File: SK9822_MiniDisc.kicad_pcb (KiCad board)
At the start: 2 copper layers, 210 x 210 mm, 331 parts

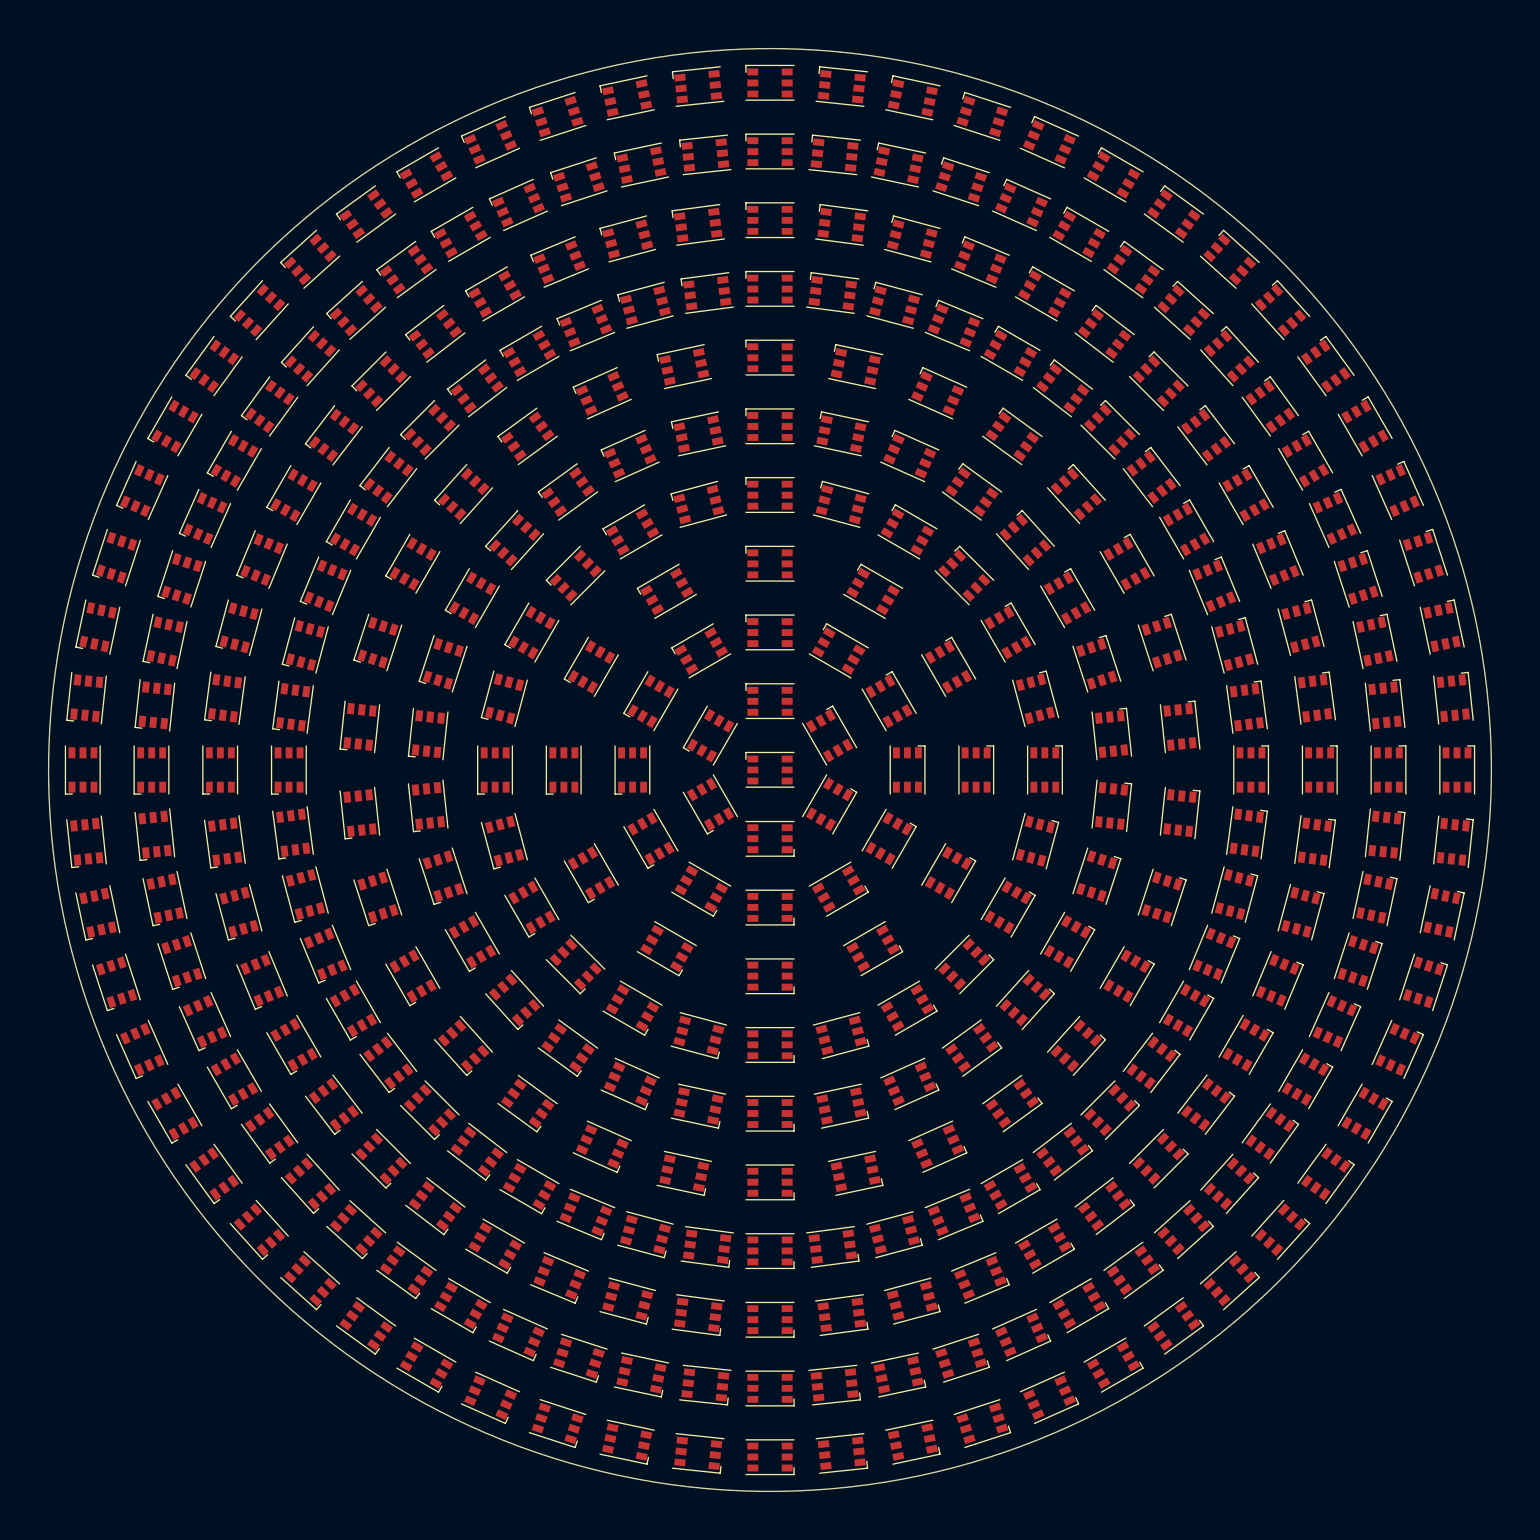
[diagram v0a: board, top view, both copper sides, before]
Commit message: Complete signal routing. Power needed
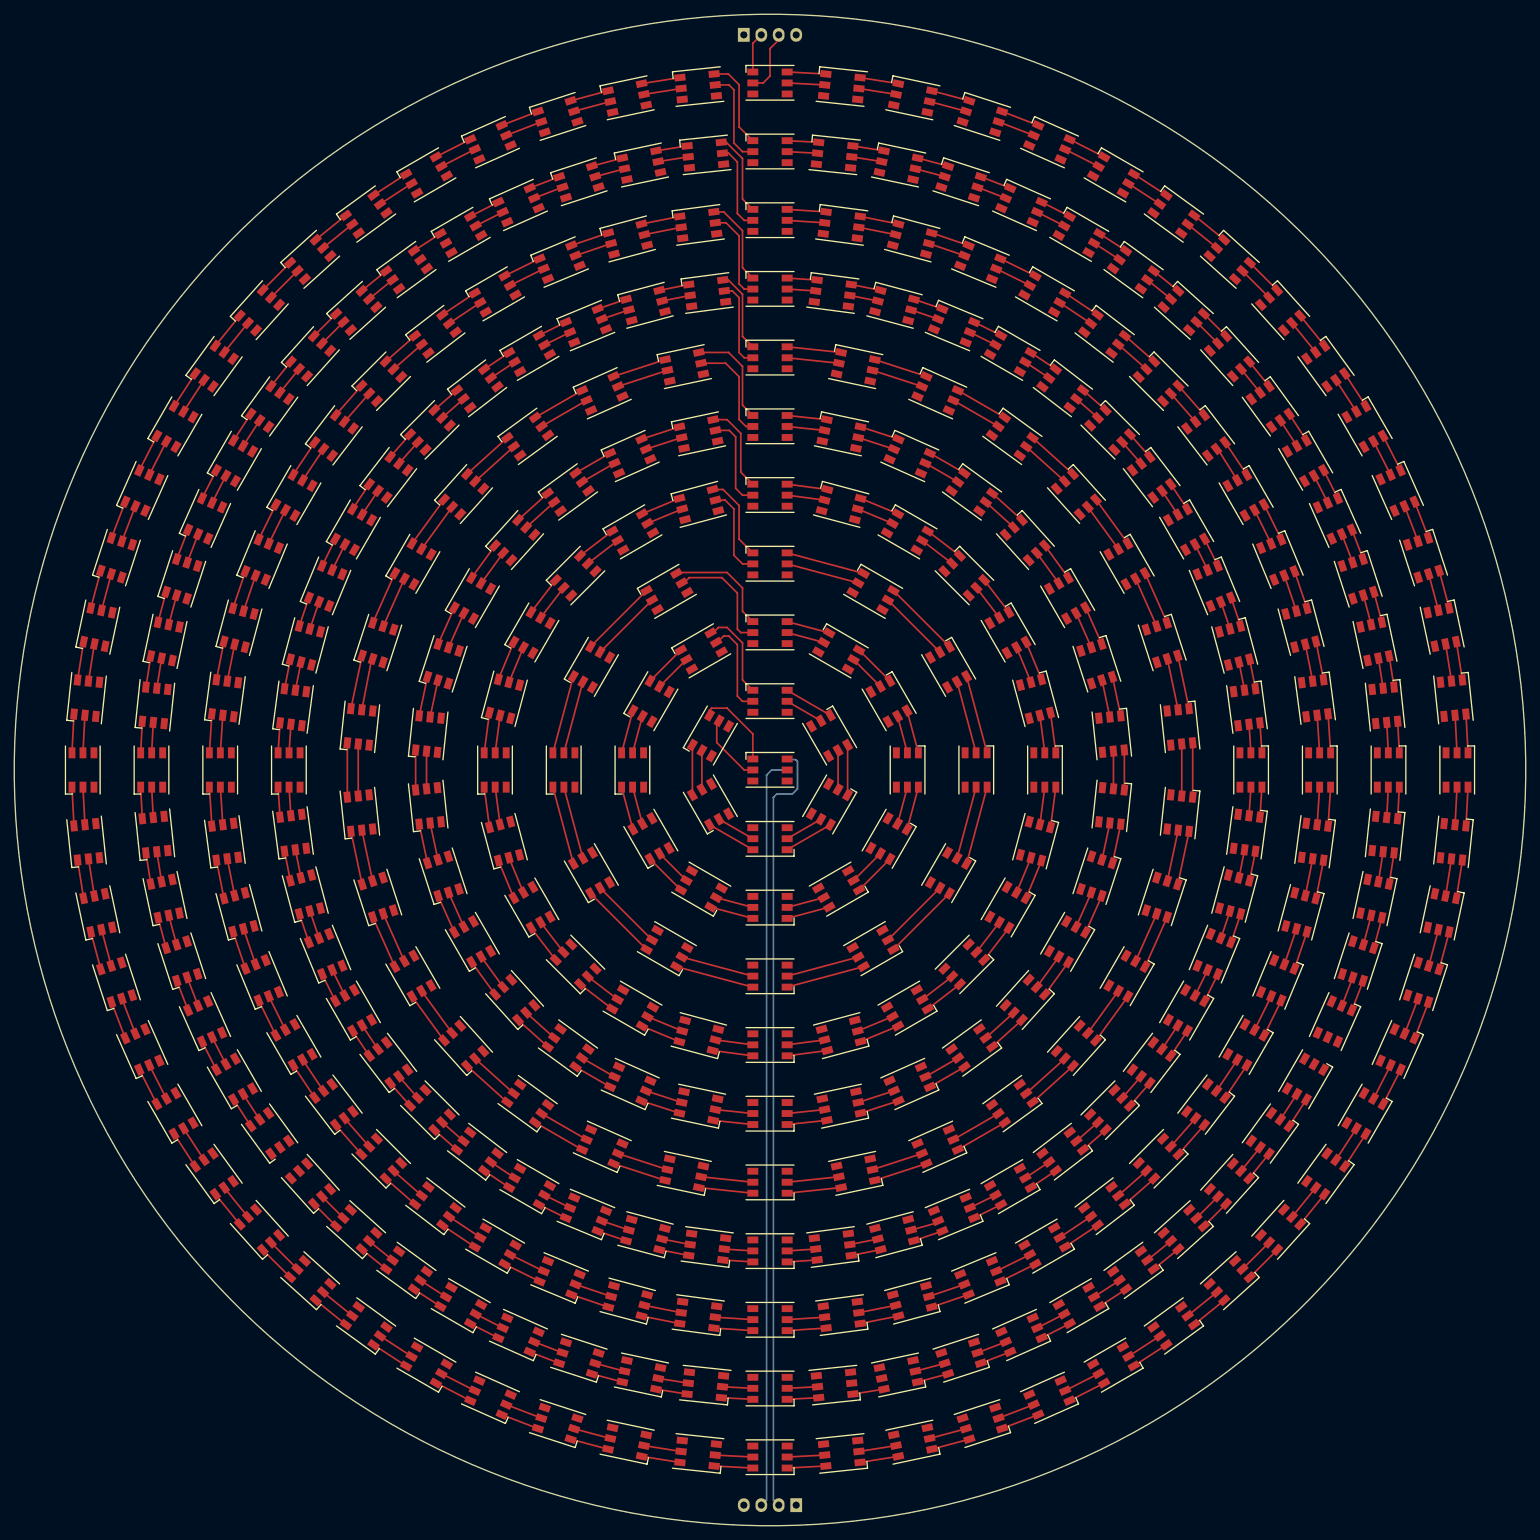
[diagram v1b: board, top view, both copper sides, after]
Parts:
- added P1: CONN_01X04, Conn:Angled_1x4, B.Cu at (300.0, 93.0)
- added P2: CONN_01X04, Conn:Angled_1x4, B.Cu at (300.0, 307.0)
- D1, D10, D100, D101, D102, D103, D104, D105, D106, D107, D108, D109, D11, D110, D111, D112, D113, D114, D115, D116, D117, D118, D119, D12, D120, D121, D122, D123, D124, D125, D126, D127, D128, D129, D13, D130, D131, D132, D133, D134, D135, D136, D137, D138, D139, D14, D140, D141, D142, D143, D144, D145, D146, D147, D148, D149, D15, D150, D151, D152, D153, D154, D155, D156, D157, D158, D159, D16, D160, D161, D162, D163, D164, D165, D166, D167, D168, D169, D17, D170, D171, D172, D173, D174, D175, D176, D177, D178, D179, D18, D180, D181, D182, D183, D184, D185, D186, D187, D188, D189, D19, D190, D191, D192, D193, D194, D195, D196, D197, D198, D199, D2, D20, D200, D201, D202, D203, D204, D205, D206, D207, D208, D209, D21, D210, D211, D212, D213, D214, D215, D216, D217, D218, D219, D22, D220, D221, D222, D223, D224, D225, D226, D227, D228, D229, D23, D230, D231, D232, D233, D234, D235, D236, D237, D238, D239, D24, D240, D241, D242, D243, D244, D245, D246, D247, D248, D249, D25, D250, D251, D252, D253, D254, D255, D256, D257, D258, D259, D26, D260, D261, D262, D263, D264, D265, D266, D267, D268, D269, D27, D270, D271, D272, D273, D274, D275, D276, D277, D278, D279, D28, D280, D281, D282, D283, D284, D285, D286, D287, D288, D289, D29, D290, D291, D292, D293, D294, D295, D296, D297, D298, D299, D3, D30, D300, D301, D302, D303, D304, D305, D306, D307, D308, D309, D31, D310, D311, D312, D313, D314, D315, D316, D317, D318, D319, D32, D320, D321, D322, D323, D324, D325, D326, D327, D328, D329, D33, D330, D331, D34, D35, D36, D37, D38, D39, D4, D40, D41, D42, D43, D44, D45, D46, D47, D48, D49, D5, D50, D51, D52, D53, D54, D55, D56, D57, D58, D59, D6, D60, D61, D62, D63, D64, D65, D66, D67, D68, D69, D7, D70, D71, D72, D73, D74, D75, D76, D77, D78, D79, D8, D80, D81, D82, D83, D84, D85, D86, D87, D88, D89, D9, D90, D91, D92, D93, D94, D95, D96, D97, D98, D99: value SK9822 -> APA102/SK9822
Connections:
- D1 pad 1: (no net) -> Net-(D1-Pad1)
- D1 pad 2: (no net) -> Net-(D1-Pad2)
- D1 pad 3: (no net) -> GND
- D1 pad 4: (no net) -> VCC
- D1 pad 5: (no net) -> Net-(D1-Pad5)
- D1 pad 6: (no net) -> Net-(D1-Pad6)
- D10 pad 1: (no net) -> Net-(D10-Pad1)
- D10 pad 2: (no net) -> Net-(D10-Pad2)
- D10 pad 3: (no net) -> GND
- D10 pad 4: (no net) -> VCC
- D10 pad 5: (no net) -> Net-(D10-Pad5)
- D10 pad 6: (no net) -> Net-(D10-Pad6)
- D100 pad 1: (no net) -> Net-(D100-Pad1)
- D100 pad 2: (no net) -> Net-(D100-Pad2)
- D100 pad 3: (no net) -> GND
- D100 pad 4: (no net) -> VCC
- D100 pad 5: (no net) -> Net-(D100-Pad5)
- D100 pad 6: (no net) -> Net-(D100-Pad6)
- D101 pad 1: (no net) -> Net-(D100-Pad6)
- D101 pad 2: (no net) -> Net-(D100-Pad5)
- D101 pad 3: (no net) -> GND
- D101 pad 4: (no net) -> VCC
- D101 pad 5: (no net) -> Net-(D101-Pad5)
- D101 pad 6: (no net) -> Net-(D101-Pad6)
- D102 pad 1: (no net) -> Net-(D101-Pad6)
- D102 pad 2: (no net) -> Net-(D101-Pad5)
- D102 pad 3: (no net) -> GND
- D102 pad 4: (no net) -> VCC
- D102 pad 5: (no net) -> Net-(D102-Pad5)
- D102 pad 6: (no net) -> Net-(D102-Pad6)
- D103 pad 1: (no net) -> Net-(D102-Pad6)
- D103 pad 2: (no net) -> Net-(D102-Pad5)
- D103 pad 3: (no net) -> GND
- D103 pad 4: (no net) -> VCC
- D103 pad 5: (no net) -> Net-(D103-Pad5)
- D103 pad 6: (no net) -> Net-(D103-Pad6)
- D104 pad 1: (no net) -> Net-(D103-Pad6)
- D104 pad 2: (no net) -> Net-(D103-Pad5)
- D104 pad 3: (no net) -> GND
- D104 pad 4: (no net) -> VCC
- D104 pad 5: (no net) -> Net-(D104-Pad5)
- D104 pad 6: (no net) -> Net-(D104-Pad6)
- D105 pad 1: (no net) -> Net-(D104-Pad6)
- D105 pad 2: (no net) -> Net-(D104-Pad5)
- D105 pad 3: (no net) -> GND
- D105 pad 4: (no net) -> VCC
- D105 pad 5: (no net) -> Net-(D105-Pad5)
- D105 pad 6: (no net) -> Net-(D105-Pad6)
- D106 pad 1: (no net) -> Net-(D105-Pad6)
- D106 pad 2: (no net) -> Net-(D105-Pad5)
- D106 pad 3: (no net) -> GND
- D106 pad 4: (no net) -> VCC
- D106 pad 5: (no net) -> Net-(D106-Pad5)
- D106 pad 6: (no net) -> Net-(D106-Pad6)
- D107 pad 1: (no net) -> Net-(D106-Pad6)
- D107 pad 2: (no net) -> Net-(D106-Pad5)
- D107 pad 3: (no net) -> GND
- D107 pad 4: (no net) -> VCC
- D107 pad 5: (no net) -> Net-(D107-Pad5)
- D107 pad 6: (no net) -> Net-(D107-Pad6)
- D108 pad 1: (no net) -> Net-(D107-Pad6)
- D108 pad 2: (no net) -> Net-(D107-Pad5)
- D108 pad 3: (no net) -> GND
- D108 pad 4: (no net) -> VCC
- D108 pad 5: (no net) -> Net-(D108-Pad5)
- D108 pad 6: (no net) -> Net-(D108-Pad6)
- D109 pad 1: (no net) -> Net-(D108-Pad6)
- D109 pad 2: (no net) -> Net-(D108-Pad5)
- D109 pad 3: (no net) -> GND
- D109 pad 4: (no net) -> VCC
- D109 pad 5: (no net) -> Net-(D109-Pad5)
- D109 pad 6: (no net) -> Net-(D109-Pad6)
- D11 pad 1: (no net) -> Net-(D10-Pad6)
- D11 pad 2: (no net) -> Net-(D10-Pad5)
- D11 pad 3: (no net) -> GND
- D11 pad 4: (no net) -> VCC
- D11 pad 5: (no net) -> Net-(D11-Pad5)
- D11 pad 6: (no net) -> Net-(D11-Pad6)
- D110 pad 1: (no net) -> Net-(D109-Pad6)
- D110 pad 2: (no net) -> Net-(D109-Pad5)
- D110 pad 3: (no net) -> GND
- D110 pad 4: (no net) -> VCC
- D110 pad 5: (no net) -> Net-(D110-Pad5)
- D110 pad 6: (no net) -> Net-(D110-Pad6)
- D111 pad 1: (no net) -> Net-(D110-Pad6)
- D111 pad 2: (no net) -> Net-(D110-Pad5)
- D111 pad 3: (no net) -> GND
- D111 pad 4: (no net) -> VCC
- D111 pad 5: (no net) -> Net-(D111-Pad5)
- D111 pad 6: (no net) -> Net-(D111-Pad6)
- D112 pad 1: (no net) -> Net-(D111-Pad6)
- D112 pad 2: (no net) -> Net-(D111-Pad5)
- D112 pad 3: (no net) -> GND
- D112 pad 4: (no net) -> VCC
- D112 pad 5: (no net) -> Net-(D112-Pad5)
- D112 pad 6: (no net) -> Net-(D112-Pad6)
- D113 pad 1: (no net) -> Net-(D112-Pad6)
- D113 pad 2: (no net) -> Net-(D112-Pad5)
- D113 pad 3: (no net) -> GND
- D113 pad 4: (no net) -> VCC
- D113 pad 5: (no net) -> Net-(D113-Pad5)
- D113 pad 6: (no net) -> Net-(D113-Pad6)
- D114 pad 1: (no net) -> Net-(D113-Pad6)
- D114 pad 2: (no net) -> Net-(D113-Pad5)
- D114 pad 3: (no net) -> GND
- D114 pad 4: (no net) -> VCC
- D114 pad 5: (no net) -> Net-(D114-Pad5)
- D114 pad 6: (no net) -> Net-(D114-Pad6)
- D115 pad 1: (no net) -> Net-(D114-Pad6)
- D115 pad 2: (no net) -> Net-(D114-Pad5)
- D115 pad 3: (no net) -> GND
- D115 pad 4: (no net) -> VCC
- D115 pad 5: (no net) -> Net-(D115-Pad5)
- D115 pad 6: (no net) -> Net-(D115-Pad6)
- D116 pad 1: (no net) -> Net-(D115-Pad6)
- D116 pad 2: (no net) -> Net-(D115-Pad5)
- D116 pad 3: (no net) -> GND
- D116 pad 4: (no net) -> VCC
- D116 pad 5: (no net) -> Net-(D116-Pad5)
- D116 pad 6: (no net) -> Net-(D116-Pad6)
- D117 pad 1: (no net) -> Net-(D116-Pad6)
- D117 pad 2: (no net) -> Net-(D116-Pad5)
- D117 pad 3: (no net) -> GND
- D117 pad 4: (no net) -> VCC
- D117 pad 5: (no net) -> Net-(D117-Pad5)
- D117 pad 6: (no net) -> Net-(D117-Pad6)
- D118 pad 1: (no net) -> Net-(D117-Pad6)
- D118 pad 2: (no net) -> Net-(D117-Pad5)
- D118 pad 3: (no net) -> GND
- D118 pad 4: (no net) -> VCC
- D118 pad 5: (no net) -> Net-(D118-Pad5)
- D118 pad 6: (no net) -> Net-(D118-Pad6)
- D119 pad 1: (no net) -> Net-(D118-Pad6)
- D119 pad 2: (no net) -> Net-(D118-Pad5)
- D119 pad 3: (no net) -> GND
- D119 pad 4: (no net) -> VCC
- D119 pad 5: (no net) -> Net-(D119-Pad5)
- D119 pad 6: (no net) -> Net-(D119-Pad6)
- D12 pad 1: (no net) -> Net-(D11-Pad6)
- D12 pad 2: (no net) -> Net-(D11-Pad5)
- D12 pad 3: (no net) -> GND
- D12 pad 4: (no net) -> VCC
- D12 pad 5: (no net) -> Net-(D12-Pad5)
- D12 pad 6: (no net) -> Net-(D12-Pad6)
- D120 pad 1: (no net) -> Net-(D119-Pad6)
- D120 pad 2: (no net) -> Net-(D119-Pad5)
- D120 pad 3: (no net) -> GND
- D120 pad 4: (no net) -> VCC
- D120 pad 5: (no net) -> Net-(D120-Pad5)
- D120 pad 6: (no net) -> Net-(D120-Pad6)
- D121 pad 1: (no net) -> Net-(D120-Pad6)
- D121 pad 2: (no net) -> Net-(D120-Pad5)
- D121 pad 3: (no net) -> GND
- D121 pad 4: (no net) -> VCC
- D121 pad 5: (no net) -> Net-(D121-Pad5)
- D121 pad 6: (no net) -> Net-(D121-Pad6)
- D122 pad 1: (no net) -> Net-(D121-Pad6)
- D122 pad 2: (no net) -> Net-(D121-Pad5)
- D122 pad 3: (no net) -> GND
- D122 pad 4: (no net) -> VCC
- D122 pad 5: (no net) -> Net-(D122-Pad5)
- D122 pad 6: (no net) -> Net-(D122-Pad6)
- D123 pad 1: (no net) -> Net-(D122-Pad6)
- D123 pad 2: (no net) -> Net-(D122-Pad5)
- D123 pad 3: (no net) -> GND
- D123 pad 4: (no net) -> VCC
- D123 pad 5: (no net) -> Net-(D123-Pad5)
- D123 pad 6: (no net) -> Net-(D123-Pad6)
- D124 pad 1: (no net) -> Net-(D123-Pad6)
- D124 pad 2: (no net) -> Net-(D123-Pad5)
- D124 pad 3: (no net) -> GND
- D124 pad 4: (no net) -> VCC
- D124 pad 5: (no net) -> Net-(D124-Pad5)
- D124 pad 6: (no net) -> Net-(D124-Pad6)
- D125 pad 1: (no net) -> Net-(D124-Pad6)
- D125 pad 2: (no net) -> Net-(D124-Pad5)
- D125 pad 3: (no net) -> GND
- D125 pad 4: (no net) -> VCC
- D125 pad 5: (no net) -> Net-(D125-Pad5)
- D125 pad 6: (no net) -> Net-(D125-Pad6)
- D126 pad 1: (no net) -> Net-(D125-Pad6)
- D126 pad 2: (no net) -> Net-(D125-Pad5)
- D126 pad 3: (no net) -> GND
- D126 pad 4: (no net) -> VCC
- D126 pad 5: (no net) -> Net-(D126-Pad5)
- D126 pad 6: (no net) -> Net-(D126-Pad6)
- D127 pad 1: (no net) -> Net-(D126-Pad6)
- D127 pad 2: (no net) -> Net-(D126-Pad5)
- D127 pad 3: (no net) -> GND
- D127 pad 4: (no net) -> VCC
- D127 pad 5: (no net) -> Net-(D127-Pad5)
- D127 pad 6: (no net) -> Net-(D127-Pad6)
- D128 pad 1: (no net) -> Net-(D127-Pad6)
- D128 pad 2: (no net) -> Net-(D127-Pad5)
- D128 pad 3: (no net) -> GND
- D128 pad 4: (no net) -> VCC
- D128 pad 5: (no net) -> Net-(D128-Pad5)
- D128 pad 6: (no net) -> Net-(D128-Pad6)
- D129 pad 1: (no net) -> Net-(D128-Pad6)
- D129 pad 2: (no net) -> Net-(D128-Pad5)
- D129 pad 3: (no net) -> GND
- D129 pad 4: (no net) -> VCC
- D129 pad 5: (no net) -> Net-(D129-Pad5)
- D129 pad 6: (no net) -> Net-(D129-Pad6)
- D13 pad 1: (no net) -> Net-(D12-Pad6)
- D13 pad 2: (no net) -> Net-(D12-Pad5)
- D13 pad 3: (no net) -> GND
- D13 pad 4: (no net) -> VCC
- D13 pad 5: (no net) -> Net-(D13-Pad5)
- D13 pad 6: (no net) -> Net-(D13-Pad6)
- D130 pad 1: (no net) -> Net-(D129-Pad6)
- D130 pad 2: (no net) -> Net-(D129-Pad5)
- D130 pad 3: (no net) -> GND
- D130 pad 4: (no net) -> VCC
- D130 pad 5: (no net) -> Net-(D130-Pad5)
- D130 pad 6: (no net) -> Net-(D130-Pad6)
- D131 pad 1: (no net) -> Net-(D130-Pad6)
- D131 pad 2: (no net) -> Net-(D130-Pad5)
- D131 pad 3: (no net) -> GND
- D131 pad 4: (no net) -> VCC
- D131 pad 5: (no net) -> Net-(D131-Pad5)
- D131 pad 6: (no net) -> Net-(D131-Pad6)
- D132 pad 1: (no net) -> Net-(D131-Pad6)
- D132 pad 2: (no net) -> Net-(D131-Pad5)
- D132 pad 3: (no net) -> GND
- D132 pad 4: (no net) -> VCC
- D132 pad 5: (no net) -> Net-(D132-Pad5)
- D132 pad 6: (no net) -> Net-(D132-Pad6)
- D133 pad 1: (no net) -> Net-(D132-Pad6)
- D133 pad 2: (no net) -> Net-(D132-Pad5)
- D133 pad 3: (no net) -> GND
- D133 pad 4: (no net) -> VCC
- D133 pad 5: (no net) -> Net-(D133-Pad5)
- D133 pad 6: (no net) -> Net-(D133-Pad6)
- D134 pad 1: (no net) -> Net-(D133-Pad6)
- D134 pad 2: (no net) -> Net-(D133-Pad5)
- D134 pad 3: (no net) -> GND
- D134 pad 4: (no net) -> VCC
- D134 pad 5: (no net) -> Net-(D134-Pad5)
- D134 pad 6: (no net) -> Net-(D134-Pad6)
- D135 pad 1: (no net) -> Net-(D134-Pad6)
- D135 pad 2: (no net) -> Net-(D134-Pad5)
- D135 pad 3: (no net) -> GND
- D135 pad 4: (no net) -> VCC
- D135 pad 5: (no net) -> Net-(D135-Pad5)
- D135 pad 6: (no net) -> Net-(D135-Pad6)
- D136 pad 1: (no net) -> Net-(D135-Pad6)
- D136 pad 2: (no net) -> Net-(D135-Pad5)
- D136 pad 3: (no net) -> GND
- D136 pad 4: (no net) -> VCC
- D136 pad 5: (no net) -> Net-(D136-Pad5)
- D136 pad 6: (no net) -> Net-(D136-Pad6)
- D137 pad 1: (no net) -> Net-(D136-Pad6)
- D137 pad 2: (no net) -> Net-(D136-Pad5)
- D137 pad 3: (no net) -> GND
- D137 pad 4: (no net) -> VCC
- D137 pad 5: (no net) -> Net-(D137-Pad5)
- D137 pad 6: (no net) -> Net-(D137-Pad6)
- D138 pad 1: (no net) -> Net-(D137-Pad6)
- D138 pad 2: (no net) -> Net-(D137-Pad5)
- D138 pad 3: (no net) -> GND
- D138 pad 4: (no net) -> VCC
- D138 pad 5: (no net) -> Net-(D138-Pad5)
- D138 pad 6: (no net) -> Net-(D138-Pad6)
- D139 pad 1: (no net) -> Net-(D138-Pad6)
- D139 pad 2: (no net) -> Net-(D138-Pad5)
- D139 pad 3: (no net) -> GND
- D139 pad 4: (no net) -> VCC
- D139 pad 5: (no net) -> Net-(D139-Pad5)
- D139 pad 6: (no net) -> Net-(D139-Pad6)
- D14 pad 1: (no net) -> Net-(D13-Pad6)
- D14 pad 2: (no net) -> Net-(D13-Pad5)
- D14 pad 3: (no net) -> GND
- D14 pad 4: (no net) -> VCC
- D14 pad 5: (no net) -> Net-(D14-Pad5)
- D14 pad 6: (no net) -> Net-(D14-Pad6)
- D140 pad 1: (no net) -> Net-(D139-Pad6)
- D140 pad 2: (no net) -> Net-(D139-Pad5)
- D140 pad 3: (no net) -> GND
- D140 pad 4: (no net) -> VCC
- D140 pad 5: (no net) -> Net-(D140-Pad5)
- D140 pad 6: (no net) -> Net-(D140-Pad6)
- D141 pad 1: (no net) -> Net-(D140-Pad6)
- D141 pad 2: (no net) -> Net-(D140-Pad5)
- D141 pad 3: (no net) -> GND
- D141 pad 4: (no net) -> VCC
- D141 pad 5: (no net) -> Net-(D141-Pad5)
- D141 pad 6: (no net) -> Net-(D141-Pad6)
- D142 pad 1: (no net) -> Net-(D141-Pad6)
- D142 pad 2: (no net) -> Net-(D141-Pad5)
- D142 pad 3: (no net) -> GND
- D142 pad 4: (no net) -> VCC
- D142 pad 5: (no net) -> Net-(D142-Pad5)
- D142 pad 6: (no net) -> Net-(D142-Pad6)
- D143 pad 1: (no net) -> Net-(D142-Pad6)
- D143 pad 2: (no net) -> Net-(D142-Pad5)
- D143 pad 3: (no net) -> GND
- D143 pad 4: (no net) -> VCC
- D143 pad 5: (no net) -> Net-(D143-Pad5)
- D143 pad 6: (no net) -> Net-(D143-Pad6)
- D144 pad 1: (no net) -> Net-(D143-Pad6)
- D144 pad 2: (no net) -> Net-(D143-Pad5)
- D144 pad 3: (no net) -> GND
- D144 pad 4: (no net) -> VCC
- D144 pad 5: (no net) -> Net-(D144-Pad5)
- D144 pad 6: (no net) -> Net-(D144-Pad6)
- D145 pad 1: (no net) -> Net-(D144-Pad6)
- D145 pad 2: (no net) -> Net-(D144-Pad5)
- D145 pad 3: (no net) -> GND
- D145 pad 4: (no net) -> VCC
- D145 pad 5: (no net) -> Net-(D145-Pad5)
- D145 pad 6: (no net) -> Net-(D145-Pad6)
- D146 pad 1: (no net) -> Net-(D145-Pad6)
- D146 pad 2: (no net) -> Net-(D145-Pad5)
- D146 pad 3: (no net) -> GND
- D146 pad 4: (no net) -> VCC
- D146 pad 5: (no net) -> Net-(D146-Pad5)
- D146 pad 6: (no net) -> Net-(D146-Pad6)
- D147 pad 1: (no net) -> Net-(D146-Pad6)
- D147 pad 2: (no net) -> Net-(D146-Pad5)
- D147 pad 3: (no net) -> GND
- D147 pad 4: (no net) -> VCC
- D147 pad 5: (no net) -> Net-(D147-Pad5)
- D147 pad 6: (no net) -> Net-(D147-Pad6)
- D148 pad 1: (no net) -> Net-(D147-Pad6)
- D148 pad 2: (no net) -> Net-(D147-Pad5)
- D148 pad 3: (no net) -> GND
- D148 pad 4: (no net) -> VCC
- D148 pad 5: (no net) -> Net-(D148-Pad5)
- D148 pad 6: (no net) -> Net-(D148-Pad6)
- D149 pad 1: (no net) -> Net-(D148-Pad6)
- D149 pad 2: (no net) -> Net-(D148-Pad5)
- D149 pad 3: (no net) -> GND
- D149 pad 4: (no net) -> VCC
- D149 pad 5: (no net) -> Net-(D149-Pad5)
- D149 pad 6: (no net) -> Net-(D149-Pad6)
- D15 pad 1: (no net) -> Net-(D14-Pad6)
- D15 pad 2: (no net) -> Net-(D14-Pad5)
- D15 pad 3: (no net) -> GND
- D15 pad 4: (no net) -> VCC
- D15 pad 5: (no net) -> Net-(D15-Pad5)
- D15 pad 6: (no net) -> Net-(D15-Pad6)
- D150 pad 1: (no net) -> Net-(D149-Pad6)
- D150 pad 2: (no net) -> Net-(D149-Pad5)
- D150 pad 3: (no net) -> GND
- D150 pad 4: (no net) -> VCC
- D150 pad 5: (no net) -> Net-(D150-Pad5)
- D150 pad 6: (no net) -> Net-(D150-Pad6)
- D151 pad 1: (no net) -> Net-(D150-Pad6)
- D151 pad 2: (no net) -> Net-(D150-Pad5)
- D151 pad 3: (no net) -> GND
- D151 pad 4: (no net) -> VCC
- D151 pad 5: (no net) -> Net-(D151-Pad5)
- D151 pad 6: (no net) -> Net-(D151-Pad6)
- D152 pad 1: (no net) -> Net-(D151-Pad6)
- D152 pad 2: (no net) -> Net-(D151-Pad5)
- D152 pad 3: (no net) -> GND
- D152 pad 4: (no net) -> VCC
- D152 pad 5: (no net) -> Net-(D152-Pad5)
- D152 pad 6: (no net) -> Net-(D152-Pad6)
- D153 pad 1: (no net) -> Net-(D152-Pad6)
- D153 pad 2: (no net) -> Net-(D152-Pad5)
- D153 pad 3: (no net) -> GND
- D153 pad 4: (no net) -> VCC
- D153 pad 5: (no net) -> Net-(D153-Pad5)
- D153 pad 6: (no net) -> Net-(D153-Pad6)
- D154 pad 1: (no net) -> Net-(D153-Pad6)
- D154 pad 2: (no net) -> Net-(D153-Pad5)
- D154 pad 3: (no net) -> GND
- D154 pad 4: (no net) -> VCC
- D154 pad 5: (no net) -> Net-(D154-Pad5)
- D154 pad 6: (no net) -> Net-(D154-Pad6)
- D155 pad 1: (no net) -> Net-(D154-Pad6)
- D155 pad 2: (no net) -> Net-(D154-Pad5)
- D155 pad 3: (no net) -> GND
- D155 pad 4: (no net) -> VCC
- D155 pad 5: (no net) -> Net-(D155-Pad5)
- D155 pad 6: (no net) -> Net-(D155-Pad6)
- D156 pad 1: (no net) -> Net-(D155-Pad6)
- D156 pad 2: (no net) -> Net-(D155-Pad5)
- D156 pad 3: (no net) -> GND
- D156 pad 4: (no net) -> VCC
- D156 pad 5: (no net) -> Net-(D156-Pad5)
- D156 pad 6: (no net) -> Net-(D156-Pad6)
- D157 pad 1: (no net) -> Net-(D156-Pad6)
- D157 pad 2: (no net) -> Net-(D156-Pad5)
- D157 pad 3: (no net) -> GND
- D157 pad 4: (no net) -> VCC
- D157 pad 5: (no net) -> Net-(D157-Pad5)
- D157 pad 6: (no net) -> Net-(D157-Pad6)
- D158 pad 1: (no net) -> Net-(D157-Pad6)
- D158 pad 2: (no net) -> Net-(D157-Pad5)
- D158 pad 3: (no net) -> GND
- D158 pad 4: (no net) -> VCC
- D158 pad 5: (no net) -> Net-(D158-Pad5)
- D158 pad 6: (no net) -> Net-(D158-Pad6)
- D159 pad 1: (no net) -> Net-(D158-Pad6)
- D159 pad 2: (no net) -> Net-(D158-Pad5)
- D159 pad 3: (no net) -> GND
- D159 pad 4: (no net) -> VCC
- D159 pad 5: (no net) -> Net-(D159-Pad5)
- D159 pad 6: (no net) -> Net-(D159-Pad6)
- D16 pad 1: (no net) -> Net-(D15-Pad6)
- D16 pad 2: (no net) -> Net-(D15-Pad5)
- D16 pad 3: (no net) -> GND
- D16 pad 4: (no net) -> VCC
- D16 pad 5: (no net) -> Net-(D16-Pad5)
- D16 pad 6: (no net) -> Net-(D16-Pad6)
- D160 pad 1: (no net) -> Net-(D159-Pad6)
- D160 pad 2: (no net) -> Net-(D159-Pad5)
- D160 pad 3: (no net) -> GND
- D160 pad 4: (no net) -> VCC
- D160 pad 5: (no net) -> Net-(D160-Pad5)
- D160 pad 6: (no net) -> Net-(D160-Pad6)
- D161 pad 1: (no net) -> Net-(D160-Pad6)
- D161 pad 2: (no net) -> Net-(D160-Pad5)
- D161 pad 3: (no net) -> GND
- D161 pad 4: (no net) -> VCC
- D161 pad 5: (no net) -> Net-(D161-Pad5)
- D161 pad 6: (no net) -> Net-(D161-Pad6)
- D162 pad 1: (no net) -> Net-(D161-Pad6)
- D162 pad 2: (no net) -> Net-(D161-Pad5)
- D162 pad 3: (no net) -> GND
- D162 pad 4: (no net) -> VCC
- D162 pad 5: (no net) -> Net-(D162-Pad5)
- D162 pad 6: (no net) -> Net-(D162-Pad6)
- D163 pad 1: (no net) -> Net-(D162-Pad6)
- D163 pad 2: (no net) -> Net-(D162-Pad5)
- D163 pad 3: (no net) -> GND
- D163 pad 4: (no net) -> VCC
- D163 pad 5: (no net) -> Net-(D163-Pad5)
- D163 pad 6: (no net) -> Net-(D163-Pad6)
- D164 pad 1: (no net) -> Net-(D163-Pad6)
- D164 pad 2: (no net) -> Net-(D163-Pad5)
- D164 pad 3: (no net) -> GND
- D164 pad 4: (no net) -> VCC
- D164 pad 5: (no net) -> Net-(D164-Pad5)
- D164 pad 6: (no net) -> Net-(D164-Pad6)
- D165 pad 1: (no net) -> Net-(D164-Pad6)
- D165 pad 2: (no net) -> Net-(D164-Pad5)
- D165 pad 3: (no net) -> GND
- D165 pad 4: (no net) -> VCC
- D165 pad 5: (no net) -> Net-(D165-Pad5)
- D165 pad 6: (no net) -> Net-(D165-Pad6)
- D166 pad 1: (no net) -> Net-(D165-Pad6)
- D166 pad 2: (no net) -> Net-(D165-Pad5)
- D166 pad 3: (no net) -> GND
- D166 pad 4: (no net) -> VCC
- D166 pad 5: (no net) -> Net-(D166-Pad5)
- D166 pad 6: (no net) -> Net-(D166-Pad6)
- D167 pad 1: (no net) -> Net-(D166-Pad6)
- D167 pad 2: (no net) -> Net-(D166-Pad5)
- D167 pad 3: (no net) -> GND
- D167 pad 4: (no net) -> VCC
- D167 pad 5: (no net) -> Net-(D167-Pad5)
- D167 pad 6: (no net) -> Net-(D167-Pad6)
- D168 pad 1: (no net) -> Net-(D167-Pad6)
- D168 pad 2: (no net) -> Net-(D167-Pad5)
- D168 pad 3: (no net) -> GND
- D168 pad 4: (no net) -> VCC
- D168 pad 5: (no net) -> Net-(D168-Pad5)
- D168 pad 6: (no net) -> Net-(D168-Pad6)
- D169 pad 1: (no net) -> Net-(D168-Pad6)
- D169 pad 2: (no net) -> Net-(D168-Pad5)
- D169 pad 3: (no net) -> GND
- D169 pad 4: (no net) -> VCC
- D169 pad 5: (no net) -> Net-(D169-Pad5)
- D169 pad 6: (no net) -> Net-(D169-Pad6)
- D17 pad 1: (no net) -> Net-(D16-Pad6)
- D17 pad 2: (no net) -> Net-(D16-Pad5)
- D17 pad 3: (no net) -> GND
- D17 pad 4: (no net) -> VCC
- D17 pad 5: (no net) -> Net-(D17-Pad5)
- D17 pad 6: (no net) -> Net-(D17-Pad6)
- D170 pad 1: (no net) -> Net-(D169-Pad6)
- D170 pad 2: (no net) -> Net-(D169-Pad5)
- D170 pad 3: (no net) -> GND
- D170 pad 4: (no net) -> VCC
- D170 pad 5: (no net) -> Net-(D170-Pad5)
- D170 pad 6: (no net) -> Net-(D170-Pad6)
- D171 pad 1: (no net) -> Net-(D170-Pad6)
- D171 pad 2: (no net) -> Net-(D170-Pad5)
- D171 pad 3: (no net) -> GND
- D171 pad 4: (no net) -> VCC
- D171 pad 5: (no net) -> Net-(D171-Pad5)
- D171 pad 6: (no net) -> Net-(D171-Pad6)
- D172 pad 1: (no net) -> Net-(D171-Pad6)
- D172 pad 2: (no net) -> Net-(D171-Pad5)
- D172 pad 3: (no net) -> GND
- D172 pad 4: (no net) -> VCC
- D172 pad 5: (no net) -> Net-(D172-Pad5)
- D172 pad 6: (no net) -> Net-(D172-Pad6)
- D173 pad 1: (no net) -> Net-(D172-Pad6)
- D173 pad 2: (no net) -> Net-(D172-Pad5)
- D173 pad 3: (no net) -> GND
- D173 pad 4: (no net) -> VCC
- D173 pad 5: (no net) -> Net-(D173-Pad5)
- D173 pad 6: (no net) -> Net-(D173-Pad6)
- D174 pad 1: (no net) -> Net-(D173-Pad6)
- D174 pad 2: (no net) -> Net-(D173-Pad5)
- D174 pad 3: (no net) -> GND
- D174 pad 4: (no net) -> VCC
- D174 pad 5: (no net) -> Net-(D174-Pad5)
- D174 pad 6: (no net) -> Net-(D174-Pad6)
- D175 pad 1: (no net) -> Net-(D174-Pad6)
- D175 pad 2: (no net) -> Net-(D174-Pad5)
- D175 pad 3: (no net) -> GND
- D175 pad 4: (no net) -> VCC
- D175 pad 5: (no net) -> Net-(D175-Pad5)
- D175 pad 6: (no net) -> Net-(D175-Pad6)
- D176 pad 1: (no net) -> Net-(D175-Pad6)
- D176 pad 2: (no net) -> Net-(D175-Pad5)
- D176 pad 3: (no net) -> GND
- D176 pad 4: (no net) -> VCC
- D176 pad 5: (no net) -> Net-(D176-Pad5)
- D176 pad 6: (no net) -> Net-(D176-Pad6)
- D177 pad 1: (no net) -> Net-(D176-Pad6)
- D177 pad 2: (no net) -> Net-(D176-Pad5)
- D177 pad 3: (no net) -> GND
- D177 pad 4: (no net) -> VCC
- D177 pad 5: (no net) -> Net-(D177-Pad5)
- D177 pad 6: (no net) -> Net-(D177-Pad6)
- D178 pad 1: (no net) -> Net-(D177-Pad6)
- D178 pad 2: (no net) -> Net-(D177-Pad5)
- D178 pad 3: (no net) -> GND
- D178 pad 4: (no net) -> VCC
- D178 pad 5: (no net) -> Net-(D178-Pad5)
- D178 pad 6: (no net) -> Net-(D178-Pad6)
- D179 pad 1: (no net) -> Net-(D178-Pad6)
- D179 pad 2: (no net) -> Net-(D178-Pad5)
- D179 pad 3: (no net) -> GND
- D179 pad 4: (no net) -> VCC
- D179 pad 5: (no net) -> Net-(D179-Pad5)
- D179 pad 6: (no net) -> Net-(D179-Pad6)
- D18 pad 1: (no net) -> Net-(D17-Pad6)
- D18 pad 2: (no net) -> Net-(D17-Pad5)
- D18 pad 3: (no net) -> GND
- D18 pad 4: (no net) -> VCC
- D18 pad 5: (no net) -> Net-(D18-Pad5)
- D18 pad 6: (no net) -> Net-(D18-Pad6)
- D180 pad 1: (no net) -> Net-(D179-Pad6)
- D180 pad 2: (no net) -> Net-(D179-Pad5)
- D180 pad 3: (no net) -> GND
- D180 pad 4: (no net) -> VCC
- D180 pad 5: (no net) -> Net-(D180-Pad5)
- D180 pad 6: (no net) -> Net-(D180-Pad6)
- D181 pad 1: (no net) -> Net-(D180-Pad6)
- D181 pad 2: (no net) -> Net-(D180-Pad5)
- D181 pad 3: (no net) -> GND
- D181 pad 4: (no net) -> VCC
- D181 pad 5: (no net) -> Net-(D181-Pad5)
- D181 pad 6: (no net) -> Net-(D181-Pad6)
- D182 pad 1: (no net) -> Net-(D181-Pad6)
- D182 pad 2: (no net) -> Net-(D181-Pad5)
- D182 pad 3: (no net) -> GND
- D182 pad 4: (no net) -> VCC
- D182 pad 5: (no net) -> Net-(D182-Pad5)
- D182 pad 6: (no net) -> Net-(D182-Pad6)
- D183 pad 1: (no net) -> Net-(D182-Pad6)
- D183 pad 2: (no net) -> Net-(D182-Pad5)
- D183 pad 3: (no net) -> GND
- D183 pad 4: (no net) -> VCC
- D183 pad 5: (no net) -> Net-(D183-Pad5)
- D183 pad 6: (no net) -> Net-(D183-Pad6)
- D184 pad 1: (no net) -> Net-(D183-Pad6)
- D184 pad 2: (no net) -> Net-(D183-Pad5)
- D184 pad 3: (no net) -> GND
- D184 pad 4: (no net) -> VCC
- D184 pad 5: (no net) -> Net-(D184-Pad5)
- D184 pad 6: (no net) -> Net-(D184-Pad6)
- D185 pad 1: (no net) -> Net-(D184-Pad6)
- D185 pad 2: (no net) -> Net-(D184-Pad5)
- D185 pad 3: (no net) -> GND
- D185 pad 4: (no net) -> VCC
- D185 pad 5: (no net) -> Net-(D185-Pad5)
- D185 pad 6: (no net) -> Net-(D185-Pad6)
- D186 pad 1: (no net) -> Net-(D185-Pad6)
- D186 pad 2: (no net) -> Net-(D185-Pad5)
- D186 pad 3: (no net) -> GND
- D186 pad 4: (no net) -> VCC
- D186 pad 5: (no net) -> Net-(D186-Pad5)
- D186 pad 6: (no net) -> Net-(D186-Pad6)
- D187 pad 1: (no net) -> Net-(D186-Pad6)
- D187 pad 2: (no net) -> Net-(D186-Pad5)
- D187 pad 3: (no net) -> GND
- D187 pad 4: (no net) -> VCC
- D187 pad 5: (no net) -> Net-(D187-Pad5)
- D187 pad 6: (no net) -> Net-(D187-Pad6)
- D188 pad 1: (no net) -> Net-(D187-Pad6)
- D188 pad 2: (no net) -> Net-(D187-Pad5)
- D188 pad 3: (no net) -> GND
- D188 pad 4: (no net) -> VCC
- D188 pad 5: (no net) -> Net-(D188-Pad5)
- D188 pad 6: (no net) -> Net-(D188-Pad6)
- D189 pad 1: (no net) -> Net-(D188-Pad6)
- D189 pad 2: (no net) -> Net-(D188-Pad5)
- D189 pad 3: (no net) -> GND
- D189 pad 4: (no net) -> VCC
- D189 pad 5: (no net) -> Net-(D189-Pad5)
- D189 pad 6: (no net) -> Net-(D189-Pad6)
- D19 pad 1: (no net) -> Net-(D18-Pad6)
- D19 pad 2: (no net) -> Net-(D18-Pad5)
- D19 pad 3: (no net) -> GND
- D19 pad 4: (no net) -> VCC
- D19 pad 5: (no net) -> Net-(D19-Pad5)
- D19 pad 6: (no net) -> Net-(D19-Pad6)
- D190 pad 1: (no net) -> Net-(D189-Pad6)
- D190 pad 2: (no net) -> Net-(D189-Pad5)
- D190 pad 3: (no net) -> GND
- D190 pad 4: (no net) -> VCC
- D190 pad 5: (no net) -> Net-(D190-Pad5)
- D190 pad 6: (no net) -> Net-(D190-Pad6)
- D191 pad 1: (no net) -> Net-(D190-Pad6)
- D191 pad 2: (no net) -> Net-(D190-Pad5)
- D191 pad 3: (no net) -> GND
- D191 pad 4: (no net) -> VCC
- D191 pad 5: (no net) -> Net-(D191-Pad5)
- D191 pad 6: (no net) -> Net-(D191-Pad6)
- D192 pad 1: (no net) -> Net-(D191-Pad6)
- D192 pad 2: (no net) -> Net-(D191-Pad5)
- D192 pad 3: (no net) -> GND
- D192 pad 4: (no net) -> VCC
- D192 pad 5: (no net) -> Net-(D192-Pad5)
- D192 pad 6: (no net) -> Net-(D192-Pad6)
- D193 pad 1: (no net) -> Net-(D192-Pad6)
- D193 pad 2: (no net) -> Net-(D192-Pad5)
- D193 pad 3: (no net) -> GND
- D193 pad 4: (no net) -> VCC
- D193 pad 5: (no net) -> Net-(D193-Pad5)
- D193 pad 6: (no net) -> Net-(D193-Pad6)
- D194 pad 1: (no net) -> Net-(D193-Pad6)
- D194 pad 2: (no net) -> Net-(D193-Pad5)
- D194 pad 3: (no net) -> GND
- D194 pad 4: (no net) -> VCC
- D194 pad 5: (no net) -> Net-(D194-Pad5)
- D194 pad 6: (no net) -> Net-(D194-Pad6)
- D195 pad 1: (no net) -> Net-(D194-Pad6)
- D195 pad 2: (no net) -> Net-(D194-Pad5)
- D195 pad 3: (no net) -> GND
- D195 pad 4: (no net) -> VCC
- D195 pad 5: (no net) -> Net-(D195-Pad5)
- D195 pad 6: (no net) -> Net-(D195-Pad6)
- D196 pad 1: (no net) -> Net-(D195-Pad6)
- D196 pad 2: (no net) -> Net-(D195-Pad5)
- D196 pad 3: (no net) -> GND
- D196 pad 4: (no net) -> VCC
- D196 pad 5: (no net) -> Net-(D196-Pad5)
- D196 pad 6: (no net) -> Net-(D196-Pad6)
- D197 pad 1: (no net) -> Net-(D196-Pad6)
- D197 pad 2: (no net) -> Net-(D196-Pad5)
- D197 pad 3: (no net) -> GND
- D197 pad 4: (no net) -> VCC
- D197 pad 5: (no net) -> Net-(D197-Pad5)
- D197 pad 6: (no net) -> Net-(D197-Pad6)
- D198 pad 1: (no net) -> Net-(D197-Pad6)
- D198 pad 2: (no net) -> Net-(D197-Pad5)
- D198 pad 3: (no net) -> GND
- D198 pad 4: (no net) -> VCC
- D198 pad 5: (no net) -> Net-(D198-Pad5)
- D198 pad 6: (no net) -> Net-(D198-Pad6)
- D199 pad 1: (no net) -> Net-(D198-Pad6)
- D199 pad 2: (no net) -> Net-(D198-Pad5)
- D199 pad 3: (no net) -> GND
- D199 pad 4: (no net) -> VCC
- D199 pad 5: (no net) -> Net-(D199-Pad5)
- D199 pad 6: (no net) -> Net-(D199-Pad6)
- D2 pad 1: (no net) -> Net-(D1-Pad6)
- D2 pad 2: (no net) -> Net-(D1-Pad5)
- D2 pad 3: (no net) -> GND
- D2 pad 4: (no net) -> VCC
- D2 pad 5: (no net) -> Net-(D2-Pad5)
- D2 pad 6: (no net) -> Net-(D2-Pad6)
- D20 pad 1: (no net) -> Net-(D19-Pad6)
- D20 pad 2: (no net) -> Net-(D19-Pad5)
- D20 pad 3: (no net) -> GND
- D20 pad 4: (no net) -> VCC
- D20 pad 5: (no net) -> Net-(D20-Pad5)
- D20 pad 6: (no net) -> Net-(D20-Pad6)
- D200 pad 1: (no net) -> Net-(D199-Pad6)
- D200 pad 2: (no net) -> Net-(D199-Pad5)
- D200 pad 3: (no net) -> GND
- D200 pad 4: (no net) -> VCC
- D200 pad 5: (no net) -> Net-(D200-Pad5)
- D200 pad 6: (no net) -> Net-(D200-Pad6)
- D201 pad 1: (no net) -> Net-(D200-Pad6)
- D201 pad 2: (no net) -> Net-(D200-Pad5)
- D201 pad 3: (no net) -> GND
- D201 pad 4: (no net) -> VCC
- D201 pad 5: (no net) -> Net-(D201-Pad5)
- D201 pad 6: (no net) -> Net-(D201-Pad6)
- D202 pad 1: (no net) -> Net-(D201-Pad6)
- D202 pad 2: (no net) -> Net-(D201-Pad5)
- D202 pad 3: (no net) -> GND
- D202 pad 4: (no net) -> VCC
- D202 pad 5: (no net) -> Net-(D202-Pad5)
- D202 pad 6: (no net) -> Net-(D202-Pad6)
- D203 pad 1: (no net) -> Net-(D202-Pad6)
- D203 pad 2: (no net) -> Net-(D202-Pad5)
- D203 pad 3: (no net) -> GND
- D203 pad 4: (no net) -> VCC
- D203 pad 5: (no net) -> Net-(D203-Pad5)
- D203 pad 6: (no net) -> Net-(D203-Pad6)
- D204 pad 1: (no net) -> Net-(D203-Pad6)
- D204 pad 2: (no net) -> Net-(D203-Pad5)
- D204 pad 3: (no net) -> GND
- D204 pad 4: (no net) -> VCC
- D204 pad 5: (no net) -> Net-(D204-Pad5)
- D204 pad 6: (no net) -> Net-(D204-Pad6)
- D205 pad 1: (no net) -> Net-(D204-Pad6)
- D205 pad 2: (no net) -> Net-(D204-Pad5)
- D205 pad 3: (no net) -> GND
- D205 pad 4: (no net) -> VCC
- D205 pad 5: (no net) -> Net-(D205-Pad5)
- D205 pad 6: (no net) -> Net-(D205-Pad6)
- D206 pad 1: (no net) -> Net-(D205-Pad6)
- D206 pad 2: (no net) -> Net-(D205-Pad5)
- D206 pad 3: (no net) -> GND
- D206 pad 4: (no net) -> VCC
- D206 pad 5: (no net) -> Net-(D206-Pad5)
- D206 pad 6: (no net) -> Net-(D206-Pad6)
- D207 pad 1: (no net) -> Net-(D206-Pad6)
- D207 pad 2: (no net) -> Net-(D206-Pad5)
- D207 pad 3: (no net) -> GND
- D207 pad 4: (no net) -> VCC
- D207 pad 5: (no net) -> Net-(D207-Pad5)
- D207 pad 6: (no net) -> Net-(D207-Pad6)
- D208 pad 1: (no net) -> Net-(D207-Pad6)
- D208 pad 2: (no net) -> Net-(D207-Pad5)
- D208 pad 3: (no net) -> GND
- D208 pad 4: (no net) -> VCC
- D208 pad 5: (no net) -> Net-(D208-Pad5)
- D208 pad 6: (no net) -> Net-(D208-Pad6)
- D209 pad 1: (no net) -> Net-(D208-Pad6)
- D209 pad 2: (no net) -> Net-(D208-Pad5)
- D209 pad 3: (no net) -> GND
- D209 pad 4: (no net) -> VCC
- D209 pad 5: (no net) -> Net-(D209-Pad5)
- D209 pad 6: (no net) -> Net-(D209-Pad6)
- D21 pad 1: (no net) -> Net-(D20-Pad6)
- D21 pad 2: (no net) -> Net-(D20-Pad5)
- D21 pad 3: (no net) -> GND
- D21 pad 4: (no net) -> VCC
- D21 pad 5: (no net) -> Net-(D21-Pad5)
- D21 pad 6: (no net) -> Net-(D21-Pad6)
- D210 pad 1: (no net) -> Net-(D209-Pad6)
- D210 pad 2: (no net) -> Net-(D209-Pad5)
- D210 pad 3: (no net) -> GND
- D210 pad 4: (no net) -> VCC
- D210 pad 5: (no net) -> Net-(D210-Pad5)
- D210 pad 6: (no net) -> Net-(D210-Pad6)
- D211 pad 1: (no net) -> Net-(D210-Pad6)
- D211 pad 2: (no net) -> Net-(D210-Pad5)
- D211 pad 3: (no net) -> GND
- D211 pad 4: (no net) -> VCC
- D211 pad 5: (no net) -> Net-(D211-Pad5)
- D211 pad 6: (no net) -> Net-(D211-Pad6)
- D212 pad 1: (no net) -> Net-(D211-Pad6)
- D212 pad 2: (no net) -> Net-(D211-Pad5)
- D212 pad 3: (no net) -> GND
- D212 pad 4: (no net) -> VCC
- D212 pad 5: (no net) -> Net-(D212-Pad5)
- D212 pad 6: (no net) -> Net-(D212-Pad6)
- D213 pad 1: (no net) -> Net-(D212-Pad6)
- D213 pad 2: (no net) -> Net-(D212-Pad5)
- D213 pad 3: (no net) -> GND
- D213 pad 4: (no net) -> VCC
- D213 pad 5: (no net) -> Net-(D213-Pad5)
- D213 pad 6: (no net) -> Net-(D213-Pad6)
- D214 pad 1: (no net) -> Net-(D213-Pad6)
- D214 pad 2: (no net) -> Net-(D213-Pad5)
- D214 pad 3: (no net) -> GND
- D214 pad 4: (no net) -> VCC
- D214 pad 5: (no net) -> Net-(D214-Pad5)
- D214 pad 6: (no net) -> Net-(D214-Pad6)
- D215 pad 1: (no net) -> Net-(D214-Pad6)
- D215 pad 2: (no net) -> Net-(D214-Pad5)
- D215 pad 3: (no net) -> GND
- D215 pad 4: (no net) -> VCC
- D215 pad 5: (no net) -> Net-(D215-Pad5)
- D215 pad 6: (no net) -> Net-(D215-Pad6)
- D216 pad 1: (no net) -> Net-(D215-Pad6)
- D216 pad 2: (no net) -> Net-(D215-Pad5)
- D216 pad 3: (no net) -> GND
- D216 pad 4: (no net) -> VCC
- D216 pad 5: (no net) -> Net-(D216-Pad5)
- D216 pad 6: (no net) -> Net-(D216-Pad6)
- D217 pad 1: (no net) -> Net-(D216-Pad6)
- D217 pad 2: (no net) -> Net-(D216-Pad5)
- D217 pad 3: (no net) -> GND
- D217 pad 4: (no net) -> VCC
- D217 pad 5: (no net) -> Net-(D217-Pad5)
- D217 pad 6: (no net) -> Net-(D217-Pad6)
- D218 pad 1: (no net) -> Net-(D217-Pad6)
- D218 pad 2: (no net) -> Net-(D217-Pad5)
- D218 pad 3: (no net) -> GND
- D218 pad 4: (no net) -> VCC
- D218 pad 5: (no net) -> Net-(D218-Pad5)
- D218 pad 6: (no net) -> Net-(D218-Pad6)
- D219 pad 1: (no net) -> Net-(D218-Pad6)
- D219 pad 2: (no net) -> Net-(D218-Pad5)
- D219 pad 3: (no net) -> GND
- D219 pad 4: (no net) -> VCC
- D219 pad 5: (no net) -> Net-(D219-Pad5)
- D219 pad 6: (no net) -> Net-(D219-Pad6)
- D22 pad 1: (no net) -> Net-(D21-Pad6)
- D22 pad 2: (no net) -> Net-(D21-Pad5)
- D22 pad 3: (no net) -> GND
- D22 pad 4: (no net) -> VCC
- D22 pad 5: (no net) -> Net-(D22-Pad5)
- D22 pad 6: (no net) -> Net-(D22-Pad6)
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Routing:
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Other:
- board size 210 x 210 mm -> 220 x 220 mm
